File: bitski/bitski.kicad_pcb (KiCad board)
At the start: 2 copper layers, 90.8 x 42.4 mm, 6 parts, among them J1 USB_C_Receptacle, U1 ESP32-S3-MINI-1-N8, U2 BQ25185, U3 XC6206PxxxMR, U4 USBLC6-2SC6

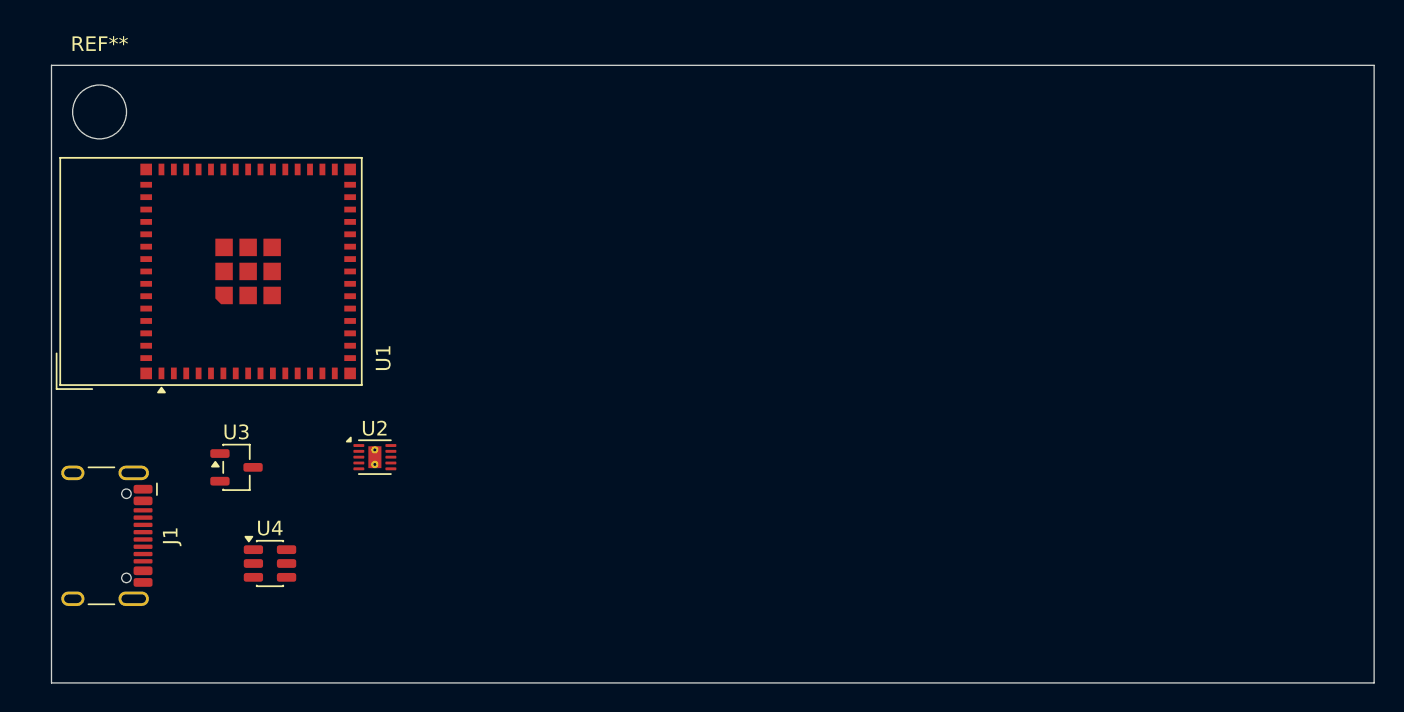
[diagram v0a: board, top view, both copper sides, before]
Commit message: made changes waow
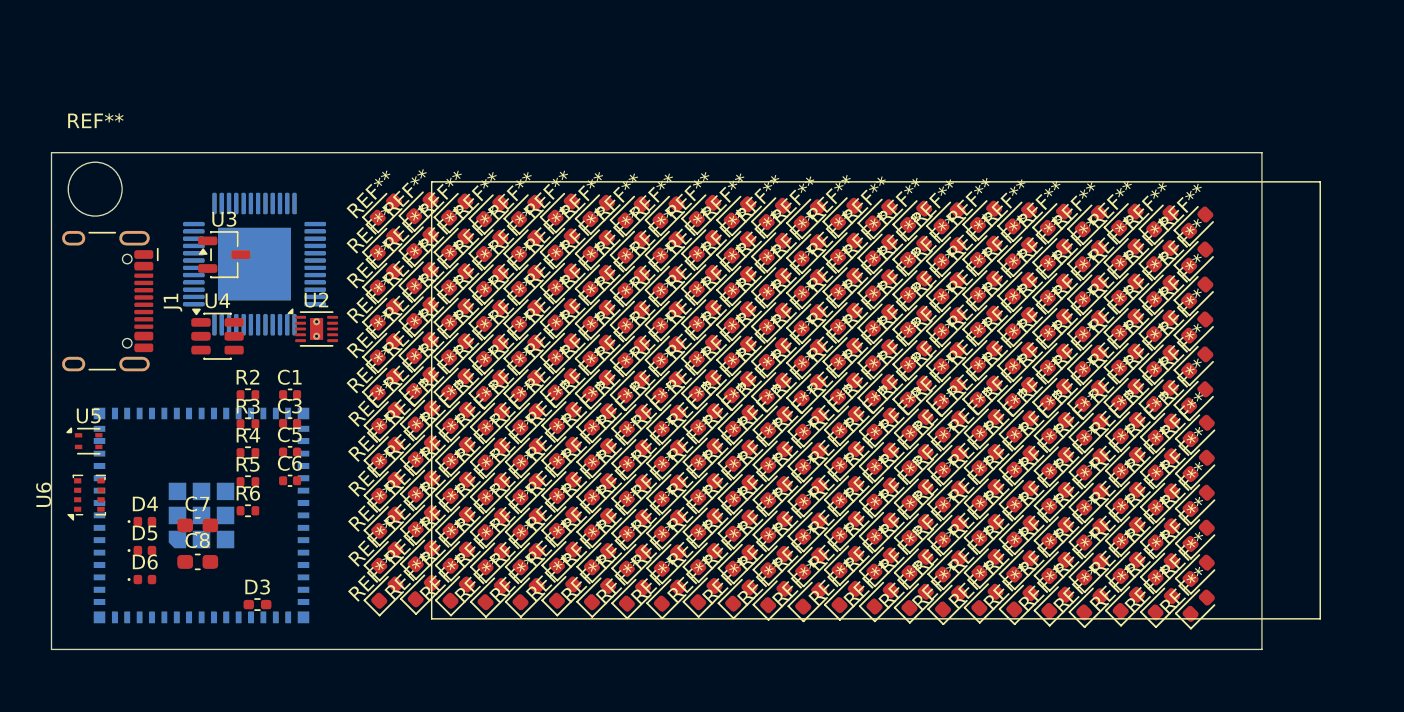
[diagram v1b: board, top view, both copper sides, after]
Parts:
- added C1: 10uF, Capacitor_SMD:C_0402_1005Metric, F.Cu at (114.0, 74.5)
- added C3: 1uF, Capacitor_SMD:C_0402_1005Metric, F.Cu at (114.0, 76.5)
- added C5: 1uF, Capacitor_SMD:C_0402_1005Metric, F.Cu at (114.0, 78.5)
- added C6: 1uF, Capacitor_SMD:C_0402_1005Metric, F.Cu at (114.0, 80.4)
- added C7: 0pF, Capacitor_SMD:C_0603_1608Metric_Pad1.08x0.95mm_HandSolder, F.Cu at (107.6, 83.5)
- added C8: 0pF, Capacitor_SMD:C_0603_1608Metric_Pad1.08x0.95mm_HandSolder, F.Cu at (107.6, 86.0)
- added D3: LED_45deg, Resistor_SMD:R_0402_1005Metric_Pad0.72x0.64mm_HandSolder, F.Cu at (111.7, 88.9)
- added D4: LED_45deg, LED_SMD:LED_0402_1005Metric, F.Cu at (104.0, 83.2)
- added D5: LED_45deg, LED_SMD:LED_0402_1005Metric, F.Cu at (104.0, 85.2)
- added D6: LED_45deg, LED_SMD:LED_0402_1005Metric, F.Cu at (104.0, 87.2)
- added R2: 5.1k, Resistor_SMD:R_0402_1005Metric, F.Cu at (111.1, 74.5)
- added R3: 5.1k, Resistor_SMD:R_0402_1005Metric, F.Cu at (111.1, 76.5)
- added R4: 10k, Resistor_SMD:R_0402_1005Metric, F.Cu at (111.1, 78.5)
- added R5: 33, Resistor_SMD:R_0402_1005Metric, F.Cu at (111.1, 80.5)
- added R6: 33, Resistor_SMD:R_0402_1005Metric, F.Cu at (111.1, 82.5)
- added REF**: LED_0603_1608Metric, LED_SMD:LED_0603_1608Metric, F.Cu at (157.0, 64.7)
- added REF**: LED_0603_1608Metric, LED_SMD:LED_0603_1608Metric, F.Cu at (154.7, 88.5)
- added REF**: LED_0603_1608Metric, LED_SMD:LED_0603_1608Metric, F.Cu at (132.8, 66.6)
- added REF**: LED_0603_1608Metric, LED_SMD:LED_0603_1608Metric, F.Cu at (169.0, 62.6)
- added REF**: LED_0603_1608Metric, LED_SMD:LED_0603_1608Metric, F.Cu at (135.3, 76.2)
- added REF**: LED_0603_1608Metric, LED_SMD:LED_0603_1608Metric, F.Cu at (147.3, 74.1)
- added REF**: LED_0603_1608Metric, LED_SMD:LED_0603_1608Metric, F.Cu at (144.9, 64.4)
- added REF**: LED_0603_1608Metric, LED_SMD:LED_0603_1608Metric, F.Cu at (120.7, 78.5)
- added REF**: LED_0603_1608Metric, LED_SMD:LED_0603_1608Metric, F.Cu at (123.2, 76.0)
- added REF**: LED_0603_1608Metric, LED_SMD:LED_0603_1608Metric, F.Cu at (152.2, 64.5)
- added REF**: LED_0603_1608Metric, LED_SMD:LED_0603_1608Metric, F.Cu at (176.3, 69.9)
- added REF**: LED_0603_1608Metric, LED_SMD:LED_0603_1608Metric, F.Cu at (152.3, 86.0)
- added REF**: LED_0603_1608Metric, LED_SMD:LED_0603_1608Metric, F.Cu at (127.9, 61.9)
- added REF**: LED_0603_1608Metric, LED_SMD:LED_0603_1608Metric, F.Cu at (176.4, 89.0)
- added REF**: LED_0603_1608Metric, LED_SMD:LED_0603_1608Metric, F.Cu at (152.2, 62.1)
- added REF**: LED_0603_1608Metric, LED_SMD:LED_0603_1608Metric, F.Cu at (169.0, 67.4)
- added REF**: LED_0603_1608Metric, LED_SMD:LED_0603_1608Metric, F.Cu at (123.2, 88.0)
- added REF**: LED_0603_1608Metric, LED_SMD:LED_0603_1608Metric, F.Cu at (169.1, 88.9)
- added REF**: LED_0603_1608Metric, LED_SMD:LED_0603_1608Metric, F.Cu at (142.5, 64.3)
- added REF**: LED_0603_1608Metric, LED_SMD:LED_0603_1608Metric, F.Cu at (154.6, 71.8)
- added REF**: LED_0603_1608Metric, LED_SMD:LED_0603_1608Metric, F.Cu at (140.1, 85.9)
- added REF**: LED_0603_1608Metric, LED_SMD:LED_0603_1608Metric, F.Cu at (142.5, 66.7)
- added REF**: LED_0603_1608Metric, LED_SMD:LED_0603_1608Metric, F.Cu at (174.0, 76.9)
- added REF**: LED_0603_1608Metric, LED_SMD:LED_0603_1608Metric, F.Cu at (137.7, 76.3)
- added REF**: LED_0603_1608Metric, LED_SMD:LED_0603_1608Metric, F.Cu at (149.7, 67.0)
- added REF**: LED_0603_1608Metric, LED_SMD:LED_0603_1608Metric, F.Cu at (142.6, 76.2)
- added REF**: LED_0603_1608Metric, LED_SMD:LED_0603_1608Metric, F.Cu at (161.8, 74.3)
- added REF**: LED_0603_1608Metric, LED_SMD:LED_0603_1608Metric, F.Cu at (125.5, 71.4)
- added REF**: LED_0603_1608Metric, LED_SMD:LED_0603_1608Metric, F.Cu at (120.6, 73.8)
- added REF**: LED_0603_1608Metric, LED_SMD:LED_0603_1608Metric, F.Cu at (164.3, 86.3)
- added REF**: LED_0603_1608Metric, LED_SMD:LED_0603_1608Metric, F.Cu at (125.6, 80.9)
- added REF**: LED_0603_1608Metric, LED_SMD:LED_0603_1608Metric, F.Cu at (145.0, 78.7)
- added REF**: LED_0603_1608Metric, LED_SMD:LED_0603_1608Metric, F.Cu at (161.8, 64.7)
- added REF**: LED_0603_1608Metric, LED_SMD:LED_0603_1608Metric, F.Cu at (159.4, 81.5)
- added REF**: LED_0603_1608Metric, LED_SMD:LED_0603_1608Metric, F.Cu at (135.2, 73.9)
- added REF**: LED_0603_1608Metric, LED_SMD:LED_0603_1608Metric, F.Cu at (166.7, 76.8)
- added REF**: LED_0603_1608Metric, LED_SMD:LED_0603_1608Metric, F.Cu at (161.8, 69.5)
- added REF**: LED_0603_1608Metric, LED_SMD:LED_0603_1608Metric, F.Cu at (171.5, 69.7)
- added REF**: LED_0603_1608Metric, LED_SMD:LED_0603_1608Metric, F.Cu at (176.3, 72.3)
- added REF**: LED_0603_1608Metric, LED_SMD:LED_0603_1608Metric, F.Cu at (123.2, 83.2)
- added REF**: LED_0603_1608Metric, LED_SMD:LED_0603_1608Metric, F.Cu at (154.7, 81.3)
- added REF**: LED_0603_1608Metric, LED_SMD:LED_0603_1608Metric, F.Cu at (161.8, 67.1)
- added REF**: LED_0603_1608Metric, LED_SMD:LED_0603_1608Metric, F.Cu at (149.7, 69.4)
- added REF**: LED_0603_1608Metric, LED_SMD:LED_0603_1608Metric, F.Cu at (142.6, 88.2)
- added REF**: LED_0603_1608Metric, LED_SMD:LED_0603_1608Metric, F.Cu at (176.3, 67.5)
- added REF**: LED_0603_1608Metric, LED_SMD:LED_0603_1608Metric, F.Cu at (157.1, 79.0)
- added REF**: LED_0603_1608Metric, LED_SMD:LED_0603_1608Metric, F.Cu at (125.6, 76.1)
- added REF**: LED_0603_1608Metric, LED_SMD:LED_0603_1608Metric, F.Cu at (176.4, 77.0)
- added REF**: LED_0603_1608Metric, LED_SMD:LED_0603_1608Metric, F.Cu at (159.4, 88.7)
- added REF**: LED_0603_1608Metric, LED_SMD:LED_0603_1608Metric, F.Cu at (137.7, 85.9)
- added REF**: LED_0603_1608Metric, LED_SMD:LED_0603_1608Metric, F.Cu at (161.8, 71.9)
- added REF**: LED_0603_1608Metric, LED_SMD:LED_0603_1608Metric, F.Cu at (144.9, 66.8)
- added REF**: LED_0603_1608Metric, LED_SMD:LED_0603_1608Metric, F.Cu at (130.3, 66.7)
- added REF**: LED_0603_1608Metric, LED_SMD:LED_0603_1608Metric, F.Cu at (144.9, 62.0)
- added REF**: LED_0603_1608Metric, LED_SMD:LED_0603_1608Metric, F.Cu at (164.2, 64.8)
- added REF**: LED_0603_1608Metric, LED_SMD:LED_0603_1608Metric, F.Cu at (140.1, 76.3)
- added REF**: LED_0603_1608Metric, LED_SMD:LED_0603_1608Metric, F.Cu at (157.1, 88.6)
- added REF**: LED_0603_1608Metric, LED_SMD:LED_0603_1608Metric, F.Cu at (123.1, 73.7)
- added REF**: LED_0603_1608Metric, LED_SMD:LED_0603_1608Metric, F.Cu at (135.3, 88.2)
- added REF**: LED_0603_1608Metric, LED_SMD:LED_0603_1608Metric, F.Cu at (135.2, 71.5)
- added REF**: LED_0603_1608Metric, LED_SMD:LED_0603_1608Metric, F.Cu at (132.9, 83.3)
- added REF**: LED_0603_1608Metric, LED_SMD:LED_0603_1608Metric, F.Cu at (171.6, 84.0)
- added REF**: LED_0603_1608Metric, LED_SMD:LED_0603_1608Metric, F.Cu at (149.8, 88.5)
- added REF**: LED_0603_1608Metric, LED_SMD:LED_0603_1608Metric, F.Cu at (174.0, 86.5)
- added REF**: LED_0603_1608Metric, LED_SMD:LED_0603_1608Metric, F.Cu at (176.3, 74.7)
- added REF**: LED_0603_1608Metric, LED_SMD:LED_0603_1608Metric, F.Cu at (132.8, 61.8)
- added REF**: LED_0603_1608Metric, LED_SMD:LED_0603_1608Metric, F.Cu at (173.9, 72.2)
- added REF**: LED_0603_1608Metric, LED_SMD:LED_0603_1608Metric, F.Cu at (145.0, 76.3)
- added REF**: LED_0603_1608Metric, LED_SMD:LED_0603_1608Metric, F.Cu at (171.6, 88.8)
- added REF**: LED_0603_1608Metric, LED_SMD:LED_0603_1608Metric, F.Cu at (169.1, 86.5)
- added REF**: LED_0603_1608Metric, LED_SMD:LED_0603_1608Metric, F.Cu at (130.4, 81.0)
- added REF**: LED_0603_1608Metric, LED_SMD:LED_0603_1608Metric, F.Cu at (164.2, 69.6)
- added REF**: LED_0603_1608Metric, LED_SMD:LED_0603_1608Metric, F.Cu at (154.7, 78.9)
- added REF**: LED_0603_1608Metric, LED_SMD:LED_0603_1608Metric, F.Cu at (137.6, 74.0)
- added REF**: LED_0603_1608Metric, LED_SMD:LED_0603_1608Metric, F.Cu at (176.3, 65.1)
- added REF**: LED_0603_1608Metric, LED_SMD:LED_0603_1608Metric, F.Cu at (147.4, 78.8)
- added REF**: LED_0603_1608Metric, LED_SMD:LED_0603_1608Metric, F.Cu at (176.4, 81.8)
- added REF**: LED_0603_1608Metric, LED_SMD:LED_0603_1608Metric, F.Cu at (173.9, 62.6)
- added REF**: LED_0603_1608Metric, LED_SMD:LED_0603_1608Metric, F.Cu at (164.3, 81.5)
- added REF**: LED_0603_1608Metric, LED_SMD:LED_0603_1608Metric, F.Cu at (137.7, 88.3)
- added REF**: LED_0603_1608Metric, LED_SMD:LED_0603_1608Metric, F.Cu at (159.3, 69.6)
- added REF**: LED_0603_1608Metric, LED_SMD:LED_0603_1608Metric, F.Cu at (135.3, 83.4)
- added REF**: LED_0603_1608Metric, LED_SMD:LED_0603_1608Metric, F.Cu at (132.9, 85.7)
- added REF**: LED_0603_1608Metric, LED_SMD:LED_0603_1608Metric, F.Cu at (135.2, 66.7)
- added REF**: LED_0603_1608Metric, LED_SMD:LED_0603_1608Metric, F.Cu at (157.1, 83.8)
- added REF**: LED_0603_1608Metric, LED_SMD:LED_0603_1608Metric, F.Cu at (157.0, 62.3)
- added REF**: LED_0603_1608Metric, LED_SMD:LED_0603_1608Metric, F.Cu at (135.2, 61.9)
- added REF**: LED_0603_1608Metric, LED_SMD:LED_0603_1608Metric, F.Cu at (166.6, 72.1)
- added REF**: LED_0603_1608Metric, LED_SMD:LED_0603_1608Metric, F.Cu at (169.0, 69.8)
- added REF**: LED_0603_1608Metric, LED_SMD:LED_0603_1608Metric, F.Cu at (173.9, 67.4)
- added REF**: LED_0603_1608Metric, LED_SMD:LED_0603_1608Metric, F.Cu at (140.0, 69.2)
- added REF**: LED_0603_1608Metric, LED_SMD:LED_0603_1608Metric, F.Cu at (120.6, 69.0)
- added REF**: LED_0603_1608Metric, LED_SMD:LED_0603_1608Metric, F.Cu at (140.0, 62.0)
- added REF**: LED_0603_1608Metric, LED_SMD:LED_0603_1608Metric, F.Cu at (142.6, 83.4)
- added REF**: LED_0603_1608Metric, LED_SMD:LED_0603_1608Metric, F.Cu at (166.6, 62.5)
- added REF**: LED_0603_1608Metric, LED_SMD:LED_0603_1608Metric, F.Cu at (164.2, 62.4)
- added REF**: LED_0603_1608Metric, LED_SMD:LED_0603_1608Metric, F.Cu at (171.6, 76.8)
- added REF**: LED_0603_1608Metric, LED_SMD:LED_0603_1608Metric, F.Cu at (142.6, 81.0)
- added REF**: LED_0603_1608Metric, LED_SMD:LED_0603_1608Metric, F.Cu at (147.4, 88.4)
- added REF**: LED_0603_1608Metric, LED_SMD:LED_0603_1608Metric, F.Cu at (128.0, 78.6)
- added REF**: LED_0603_1608Metric, LED_SMD:LED_0603_1608Metric, F.Cu at (130.4, 83.4)
- added REF**: LED_0603_1608Metric, LED_SMD:LED_0603_1608Metric, F.Cu at (120.7, 76.1)
- added REF**: LED_0603_1608Metric, LED_SMD:LED_0603_1608Metric, F.Cu at (171.5, 72.1)
- added REF**: LED_0603_1608Metric, LED_SMD:LED_0603_1608Metric, F.Cu at (159.4, 76.7)
- added REF**: LED_0603_1608Metric, LED_SMD:LED_0603_1608Metric, F.Cu at (161.9, 88.6)
- added REF**: LED_0603_1608Metric, LED_SMD:LED_0603_1608Metric, F.Cu at (171.5, 67.3)
- added REF**: LED_0603_1608Metric, LED_SMD:LED_0603_1608Metric, F.Cu at (140.0, 71.6)
- added REF**: LED_0603_1608Metric, LED_SMD:LED_0603_1608Metric, F.Cu at (125.5, 61.8)
- added REF**: LED_0603_1608Metric, LED_SMD:LED_0603_1608Metric, F.Cu at (159.4, 79.1)
- added REF**: LED_0603_1608Metric, LED_SMD:LED_0603_1608Metric, F.Cu at (174.0, 81.7)
- added REF**: LED_0603_1608Metric, LED_SMD:LED_0603_1608Metric, F.Cu at (176.4, 79.4)
- added REF**: LED_0603_1608Metric, LED_SMD:LED_0603_1608Metric, F.Cu at (130.3, 64.3)
- added REF**: LED_0603_1608Metric, LED_SMD:LED_0603_1608Metric, F.Cu at (169.1, 81.7)
- added REF**: LED_0603_1608Metric, LED_SMD:LED_0603_1608Metric, F.Cu at (130.3, 71.5)
- added REF**: LED_0603_1608Metric, LED_SMD:LED_0603_1608Metric, F.Cu at (149.8, 78.9)
- added REF**: LED_0603_1608Metric, LED_SMD:LED_0603_1608Metric, F.Cu at (127.9, 71.5)
- added REF**: LED_0603_1608Metric, LED_SMD:LED_0603_1608Metric, F.Cu at (145.0, 81.1)
- added REF**: LED_0603_1608Metric, LED_SMD:LED_0603_1608Metric, F.Cu at (166.7, 84.0)
- added REF**: LED_0603_1608Metric, LED_SMD:LED_0603_1608Metric, F.Cu at (174.0, 84.1)
- added REF**: LED_0603_1608Metric, LED_SMD:LED_0603_1608Metric, F.Cu at (135.2, 69.1)
- added REF**: LED_0603_1608Metric, LED_SMD:LED_0603_1608Metric, F.Cu at (154.6, 67.0)
- added REF**: LED_0603_1608Metric, LED_SMD:LED_0603_1608Metric, F.Cu at (154.6, 62.2)
- added REF**: LED_0603_1608Metric, LED_SMD:LED_0603_1608Metric, F.Cu at (149.7, 62.2)
- added REF**: LED_0603_1608Metric, LED_SMD:LED_0603_1608Metric, F.Cu at (132.8, 71.4)
- added REF**: LED_0603_1608Metric, LED_SMD:LED_0603_1608Metric, F.Cu at (137.7, 81.1)
- added REF**: LED_0603_1608Metric, LED_SMD:LED_0603_1608Metric, F.Cu at (157.0, 69.5)
- added REF**: LED_0603_1608Metric, LED_SMD:LED_0603_1608Metric, F.Cu at (159.3, 67.2)
- added REF**: LED_0603_1608Metric, LED_SMD:LED_0603_1608Metric, F.Cu at (130.3, 61.9)
- added REF**: LED_0603_1608Metric, LED_SMD:LED_0603_1608Metric, F.Cu at (147.4, 86.0)
- added REF**: LED_0603_1608Metric, LED_SMD:LED_0603_1608Metric, F.Cu at (125.6, 88.1)
- added REF**: LED_0603_1608Metric, LED_SMD:LED_0603_1608Metric, F.Cu at (176.3, 62.7)
- added REF**: LED_0603_1608Metric, LED_SMD:LED_0603_1608Metric, F.Cu at (164.2, 74.4)
- added REF**: LED_0603_1608Metric, LED_SMD:LED_0603_1608Metric, F.Cu at (123.1, 68.9)
- added REF**: LED_0603_1608Metric, LED_SMD:LED_0603_1608Metric, F.Cu at (171.5, 62.5)
- added REF**: LED_0603_1608Metric, LED_SMD:LED_0603_1608Metric, F.Cu at (140.0, 74.0)
- added REF**: LED_0603_1608Metric, LED_SMD:LED_0603_1608Metric, F.Cu at (169.0, 74.6)
- added REF**: LED_0603_1608Metric, LED_SMD:LED_0603_1608Metric, F.Cu at (173.9, 69.8)
- added REF**: LED_0603_1608Metric, LED_SMD:LED_0603_1608Metric, F.Cu at (169.0, 65.0)
- added REF**: LED_0603_1608Metric, LED_SMD:LED_0603_1608Metric, F.Cu at (142.5, 73.9)
- added REF**: LED_0603_1608Metric, LED_SMD:LED_0603_1608Metric, F.Cu at (125.6, 78.5)
- added REF**: LED_0603_1608Metric, LED_SMD:LED_0603_1608Metric, F.Cu at (166.6, 74.5)
- added REF**: LED_0603_1608Metric, LED_SMD:LED_0603_1608Metric, F.Cu at (169.0, 72.2)
- added REF**: LED_0603_1608Metric, LED_SMD:LED_0603_1608Metric, F.Cu at (132.8, 64.2)
- added REF**: LED_0603_1608Metric, LED_SMD:LED_0603_1608Metric, F.Cu at (174.0, 79.3)
- added REF**: LED_0603_1608Metric, LED_SMD:LED_0603_1608Metric, F.Cu at (147.4, 76.4)
- added REF**: LED_0603_1608Metric, LED_SMD:LED_0603_1608Metric, F.Cu at (147.3, 64.5)
- added REF**: LED_0603_1608Metric, LED_SMD:LED_0603_1608Metric, F.Cu at (127.9, 66.7)
- added REF**: LED_0603_1608Metric, LED_SMD:LED_0603_1608Metric, F.Cu at (120.6, 61.8)
- added REF**: LED_0603_1608Metric, LED_SMD:LED_0603_1608Metric, F.Cu at (142.5, 69.1)
- added REF**: LED_0603_1608Metric, LED_SMD:LED_0603_1608Metric, F.Cu at (169.1, 79.3)
- added REF**: LED_0603_1608Metric, LED_SMD:LED_0603_1608Metric, F.Cu at (171.5, 64.9)
- added REF**: LED_0603_1608Metric, LED_SMD:LED_0603_1608Metric, F.Cu at (130.4, 88.2)
- added REF**: LED_0603_1608Metric, LED_SMD:LED_0603_1608Metric, F.Cu at (123.2, 85.6)
- added REF**: LED_0603_1608Metric, LED_SMD:LED_0603_1608Metric, F.Cu at (149.8, 81.3)
- added REF**: LED_0603_1608Metric, LED_SMD:LED_0603_1608Metric, F.Cu at (174.0, 88.9)
- added REF**: LED_0603_1608Metric, LED_SMD:LED_0603_1608Metric, F.Cu at (154.7, 76.5)
- added REF**: LED_0603_1608Metric, LED_SMD:LED_0603_1608Metric, F.Cu at (135.3, 78.6)
- added REF**: LED_0603_1608Metric, LED_SMD:LED_0603_1608Metric, F.Cu at (157.1, 76.6)
- added REF**: LED_0603_1608Metric, LED_SMD:LED_0603_1608Metric, F.Cu at (161.9, 76.6)
- added REF**: LED_0603_1608Metric, LED_SMD:LED_0603_1608Metric, F.Cu at (137.6, 66.8)
- added REF**: LED_0603_1608Metric, LED_SMD:LED_0603_1608Metric, F.Cu at (149.7, 64.6)
- added REF**: LED_0603_1608Metric, LED_SMD:LED_0603_1608Metric, F.Cu at (147.4, 83.6)
- added REF**: LED_0603_1608Metric, LED_SMD:LED_0603_1608Metric, F.Cu at (132.9, 88.1)
- added REF**: LED_0603_1608Metric, LED_SMD:LED_0603_1608Metric, F.Cu at (142.6, 78.6)
- added REF**: LED_0603_1608Metric, LED_SMD:LED_0603_1608Metric, F.Cu at (149.8, 86.1)
- added REF**: LED_0603_1608Metric, LED_SMD:LED_0603_1608Metric, F.Cu at (142.6, 85.8)
- added REF**: LED_0603_1608Metric, LED_SMD:LED_0603_1608Metric, F.Cu at (171.5, 74.5)
- added REF**: LED_0603_1608Metric, LED_SMD:LED_0603_1608Metric, F.Cu at (123.1, 61.7)
- added REF**: LED_0603_1608Metric, LED_SMD:LED_0603_1608Metric, F.Cu at (164.3, 76.7)
- added REF**: LED_0603_1608Metric, LED_SMD:LED_0603_1608Metric, F.Cu at (159.3, 72.0)
- added REF**: LED_0603_1608Metric, LED_SMD:LED_0603_1608Metric, F.Cu at (135.2, 64.3)
- added REF**: LED_0603_1608Metric, LED_SMD:LED_0603_1608Metric, F.Cu at (128.0, 83.4)
- added REF**: LED_0603_1608Metric, LED_SMD:LED_0603_1608Metric, F.Cu at (157.0, 74.3)
- added REF**: LED_0603_1608Metric, LED_SMD:LED_0603_1608Metric, F.Cu at (159.3, 62.4)
- added REF**: LED_0603_1608Metric, LED_SMD:LED_0603_1608Metric, F.Cu at (135.3, 81.0)
- added REF**: LED_0603_1608Metric, LED_SMD:LED_0603_1608Metric, F.Cu at (125.5, 64.2)
- added REF**: LED_0603_1608Metric, LED_SMD:LED_0603_1608Metric, F.Cu at (157.1, 86.2)
- added REF**: LED_0603_1608Metric, LED_SMD:LED_0603_1608Metric, F.Cu at (140.0, 64.4)
- added REF**: LED_0603_1608Metric, LED_SMD:LED_0603_1608Metric, F.Cu at (137.7, 83.5)
- added REF**: LED_0603_1608Metric, LED_SMD:LED_0603_1608Metric, F.Cu at (140.1, 81.1)
- added REF**: LED_0603_1608Metric, LED_SMD:LED_0603_1608Metric, F.Cu at (132.8, 69.0)
- added REF**: LED_0603_1608Metric, LED_SMD:LED_0603_1608Metric, F.Cu at (149.8, 83.7)
- added REF**: LED_0603_1608Metric, LED_SMD:LED_0603_1608Metric, F.Cu at (142.5, 71.5)
- added REF**: LED_0603_1608Metric, LED_SMD:LED_0603_1608Metric, F.Cu at (152.2, 71.7)
- added REF**: LED_0603_1608Metric, LED_SMD:LED_0603_1608Metric, F.Cu at (147.3, 71.7)
- added REF**: LED_0603_1608Metric, LED_SMD:LED_0603_1608Metric, F.Cu at (152.3, 76.4)
- added REF**: LED_0603_1608Metric, LED_SMD:LED_0603_1608Metric, F.Cu at (161.9, 81.4)
- added REF**: LED_0603_1608Metric, LED_SMD:LED_0603_1608Metric, F.Cu at (166.7, 88.8)
- added REF**: LED_0603_1608Metric, LED_SMD:LED_0603_1608Metric, F.Cu at (152.3, 83.6)
- added REF**: LED_0603_1608Metric, LED_SMD:LED_0603_1608Metric, F.Cu at (154.6, 69.4)
- added REF**: LED_0603_1608Metric, LED_SMD:LED_0603_1608Metric, F.Cu at (137.6, 69.2)
- added REF**: LED_0603_1608Metric, LED_SMD:LED_0603_1608Metric, F.Cu at (149.7, 74.2)
- added REF**: LED_0603_1608Metric, LED_SMD:LED_0603_1608Metric, F.Cu at (173.9, 65.0)
- added REF**: LED_0603_1608Metric, LED_SMD:LED_0603_1608Metric, F.Cu at (157.0, 71.9)
- added REF**: LED_0603_1608Metric, LED_SMD:LED_0603_1608Metric, F.Cu at (176.4, 84.2)
- added REF**: LED_0603_1608Metric, LED_SMD:LED_0603_1608Metric, F.Cu at (120.6, 64.2)
- added REF**: LED_0603_1608Metric, LED_SMD:LED_0603_1608Metric, F.Cu at (166.6, 67.3)
- added REF**: LED_0603_1608Metric, LED_SMD:LED_0603_1608Metric, F.Cu at (152.3, 78.8)
- added REF**: LED_0603_1608Metric, LED_SMD:LED_0603_1608Metric, F.Cu at (128.0, 81.0)
- added REF**: LED_0603_1608Metric, LED_SMD:LED_0603_1608Metric, F.Cu at (144.9, 71.6)
- added REF**: LED_0603_1608Metric, LED_SMD:LED_0603_1608Metric, F.Cu at (152.3, 88.4)
- added REF**: LED_0603_1608Metric, LED_SMD:LED_0603_1608Metric, F.Cu at (159.3, 74.4)
- added REF**: LED_0603_1608Metric, LED_SMD:LED_0603_1608Metric, F.Cu at (130.4, 78.6)
- added REF**: LED_0603_1608Metric, LED_SMD:LED_0603_1608Metric, F.Cu at (145.0, 83.5)
- added REF**: LED_0603_1608Metric, LED_SMD:LED_0603_1608Metric, F.Cu at (125.5, 66.6)
- added REF**: LED_0603_1608Metric, LED_SMD:LED_0603_1608Metric, F.Cu at (120.7, 88.1)
- added REF**: LED_0603_1608Metric, LED_SMD:LED_0603_1608Metric, F.Cu at (132.9, 80.9)
- added REF**: LED_0603_1608Metric, LED_SMD:LED_0603_1608Metric, F.Cu at (149.8, 76.5)
- added REF**: LED_0603_1608Metric, LED_SMD:LED_0603_1608Metric, F.Cu at (132.8, 73.8)
- added REF**: LED_0603_1608Metric, LED_SMD:LED_0603_1608Metric, F.Cu at (137.6, 71.6)
- added REF**: LED_0603_1608Metric, LED_SMD:LED_0603_1608Metric, F.Cu at (145.0, 85.9)
- added REF**: LED_0603_1608Metric, LED_SMD:LED_0603_1608Metric, F.Cu at (152.2, 69.3)
- added REF**: LED_0603_1608Metric, LED_SMD:LED_0603_1608Metric, F.Cu at (161.9, 79.0)
- added REF**: LED_0603_1608Metric, LED_SMD:LED_0603_1608Metric, F.Cu at (140.1, 83.5)
- added REF**: LED_0603_1608Metric, LED_SMD:LED_0603_1608Metric, F.Cu at (169.1, 84.1)
- added REF**: LED_0603_1608Metric, LED_SMD:LED_0603_1608Metric, F.Cu at (166.7, 86.4)
- added REF**: LED_0603_1608Metric, LED_SMD:LED_0603_1608Metric, F.Cu at (171.6, 79.2)
- added REF**: LED_0603_1608Metric, LED_SMD:LED_0603_1608Metric, F.Cu at (152.3, 81.2)
- added REF**: LED_0603_1608Metric, LED_SMD:LED_0603_1608Metric, F.Cu at (154.7, 83.7)
- added REF**: LED_0603_1608Metric, LED_SMD:LED_0603_1608Metric, F.Cu at (135.3, 85.8)
- added REF**: LED_0603_1608Metric, LED_SMD:LED_0603_1608Metric, F.Cu at (157.0, 67.1)
- added REF**: LED_0603_1608Metric, LED_SMD:LED_0603_1608Metric, F.Cu at (147.4, 81.2)
- added REF**: LED_0603_1608Metric, LED_SMD:LED_0603_1608Metric, F.Cu at (144.9, 69.2)
- added REF**: LED_0603_1608Metric, LED_SMD:LED_0603_1608Metric, F.Cu at (164.3, 83.9)
- added REF**: LED_0603_1608Metric, LED_SMD:LED_0603_1608Metric, F.Cu at (125.6, 83.3)
- added REF**: LED_0603_1608Metric, LED_SMD:LED_0603_1608Metric, F.Cu at (152.2, 66.9)
- added REF**: LED_0603_1608Metric, LED_SMD:LED_0603_1608Metric, F.Cu at (123.1, 66.5)
- added REF**: LED_0603_1608Metric, LED_SMD:LED_0603_1608Metric, F.Cu at (166.7, 81.6)
- added REF**: LED_0603_1608Metric, LED_SMD:LED_0603_1608Metric, F.Cu at (159.4, 83.9)
- added REF**: LED_0603_1608Metric, LED_SMD:LED_0603_1608Metric, F.Cu at (147.3, 66.9)
- added REF**: LED_0603_1608Metric, LED_SMD:LED_0603_1608Metric, F.Cu at (127.9, 69.1)
- added REF**: LED_0603_1608Metric, LED_SMD:LED_0603_1608Metric, F.Cu at (130.4, 76.2)
- added REF**: LED_0603_1608Metric, LED_SMD:LED_0603_1608Metric, F.Cu at (154.6, 74.2)
- added REF**: LED_0603_1608Metric, LED_SMD:LED_0603_1608Metric, F.Cu at (145.0, 88.3)
- added REF**: LED_0603_1608Metric, LED_SMD:LED_0603_1608Metric, F.Cu at (171.6, 86.4)
- added REF**: LED_0603_1608Metric, LED_SMD:LED_0603_1608Metric, F.Cu at (173.9, 74.6)
- added REF**: LED_0603_1608Metric, LED_SMD:LED_0603_1608Metric, F.Cu at (120.7, 80.9)
- added REF**: LED_0603_1608Metric, LED_SMD:LED_0603_1608Metric, F.Cu at (127.9, 73.9)
- added REF**: LED_0603_1608Metric, LED_SMD:LED_0603_1608Metric, F.Cu at (157.1, 81.4)
- added REF**: LED_0603_1608Metric, LED_SMD:LED_0603_1608Metric, F.Cu at (147.3, 69.3)
- added REF**: LED_0603_1608Metric, LED_SMD:LED_0603_1608Metric, F.Cu at (128.0, 76.2)
- added REF**: LED_0603_1608Metric, LED_SMD:LED_0603_1608Metric, F.Cu at (140.0, 66.8)
- added REF**: LED_0603_1608Metric, LED_SMD:LED_0603_1608Metric, F.Cu at (123.2, 80.8)
- added REF**: LED_0603_1608Metric, LED_SMD:LED_0603_1608Metric, F.Cu at (130.3, 73.9)
- added REF**: LED_0603_1608Metric, LED_SMD:LED_0603_1608Metric, F.Cu at (120.7, 85.7)
- added REF**: LED_0603_1608Metric, LED_SMD:LED_0603_1608Metric, F.Cu at (140.1, 88.3)
- added REF**: LED_0603_1608Metric, LED_SMD:LED_0603_1608Metric, F.Cu at (159.3, 64.8)
- added REF**: LED_0603_1608Metric, LED_SMD:LED_0603_1608Metric, F.Cu at (127.9, 64.3)
- added REF**: LED_0603_1608Metric, LED_SMD:LED_0603_1608Metric, F.Cu at (164.3, 88.7)
- added REF**: LED_0603_1608Metric, LED_SMD:LED_0603_1608Metric, F.Cu at (132.9, 76.1)
- added REF**: LED_0603_1608Metric, LED_SMD:LED_0603_1608Metric, F.Cu at (140.1, 78.7)
- added REF**: LED_0603_1608Metric, LED_SMD:LED_0603_1608Metric, F.Cu at (137.6, 62.0)
- added REF**: LED_0603_1608Metric, LED_SMD:LED_0603_1608Metric, F.Cu at (149.7, 71.8)
- added REF**: LED_0603_1608Metric, LED_SMD:LED_0603_1608Metric, F.Cu at (166.6, 69.7)
- added REF**: LED_0603_1608Metric, LED_SMD:LED_0603_1608Metric, F.Cu at (164.3, 79.1)
- added REF**: LED_0603_1608Metric, LED_SMD:LED_0603_1608Metric, F.Cu at (154.6, 64.6)
- added REF**: LED_0603_1608Metric, LED_SMD:LED_0603_1608Metric, F.Cu at (120.6, 66.6)
- added REF**: LED_0603_1608Metric, LED_SMD:LED_0603_1608Metric, F.Cu at (125.6, 85.7)
- added REF**: LED_0603_1608Metric, LED_SMD:LED_0603_1608Metric, F.Cu at (130.4, 85.8)
- added REF**: LED_0603_1608Metric, LED_SMD:LED_0603_1608Metric, F.Cu at (128.0, 88.2)
- added REF**: LED_0603_1608Metric, LED_SMD:LED_0603_1608Metric, F.Cu at (152.2, 74.1)
- added REF**: LED_0603_1608Metric, LED_SMD:LED_0603_1608Metric, F.Cu at (120.7, 83.3)
- added REF**: LED_0603_1608Metric, LED_SMD:LED_0603_1608Metric, F.Cu at (164.2, 67.2)
- added REF**: LED_0603_1608Metric, LED_SMD:LED_0603_1608Metric, F.Cu at (161.9, 86.2)
- added REF**: LED_0603_1608Metric, LED_SMD:LED_0603_1608Metric, F.Cu at (147.3, 62.1)
- added REF**: LED_0603_1608Metric, LED_SMD:LED_0603_1608Metric, F.Cu at (125.5, 69.0)
- added REF**: LED_0603_1608Metric, LED_SMD:LED_0603_1608Metric, F.Cu at (123.1, 71.3)
- added REF**: LED_0603_1608Metric, LED_SMD:LED_0603_1608Metric, F.Cu at (176.4, 86.6)
- added REF**: LED_0603_1608Metric, LED_SMD:LED_0603_1608Metric, F.Cu at (130.3, 69.1)
- added REF**: LED_0603_1608Metric, LED_SMD:LED_0603_1608Metric, F.Cu at (154.7, 86.1)
- added REF**: LED_0603_1608Metric, LED_SMD:LED_0603_1608Metric, F.Cu at (137.6, 64.4)
- added REF**: LED_0603_1608Metric, LED_SMD:LED_0603_1608Metric, F.Cu at (128.0, 85.8)
- added REF**: LED_0603_1608Metric, LED_SMD:LED_0603_1608Metric, F.Cu at (123.2, 78.4)
- added REF**: LED_0603_1608Metric, LED_SMD:LED_0603_1608Metric, F.Cu at (161.8, 62.3)
- added REF**: LED_0603_1608Metric, LED_SMD:LED_0603_1608Metric, F.Cu at (144.9, 74.0)
- added REF**: LED_0603_1608Metric, LED_SMD:LED_0603_1608Metric, F.Cu at (159.4, 86.3)
- added REF**: LED_0603_1608Metric, LED_SMD:LED_0603_1608Metric, F.Cu at (125.5, 73.8)
- added REF**: LED_0603_1608Metric, LED_SMD:LED_0603_1608Metric, F.Cu at (137.7, 78.7)
- added REF**: LED_0603_1608Metric, LED_SMD:LED_0603_1608Metric, F.Cu at (166.6, 64.9)
- added REF**: LED_0603_1608Metric, LED_SMD:LED_0603_1608Metric, F.Cu at (132.9, 78.5)
- added REF**: LED_0603_1608Metric, LED_SMD:LED_0603_1608Metric, F.Cu at (120.6, 71.4)
- added REF**: LED_0603_1608Metric, LED_SMD:LED_0603_1608Metric, F.Cu at (171.6, 81.6)
- added REF**: LED_0603_1608Metric, LED_SMD:LED_0603_1608Metric, F.Cu at (123.1, 64.1)
- added REF**: LED_0603_1608Metric, LED_SMD:LED_0603_1608Metric, F.Cu at (166.7, 79.2)
- added REF**: LED_0603_1608Metric, LED_SMD:LED_0603_1608Metric, F.Cu at (161.9, 83.8)
- added REF**: LED_0603_1608Metric, LED_SMD:LED_0603_1608Metric, F.Cu at (142.5, 61.9)
- added REF**: LED_0603_1608Metric, LED_SMD:LED_0603_1608Metric, F.Cu at (164.2, 72.0)
- added REF**: LED_0603_1608Metric, LED_SMD:LED_0603_1608Metric, F.Cu at (169.1, 76.9)
- added U5: GXHT40AD, Sensor_Humidity:Sensirion_DFN-4_1.5x1.5mm_P0.8mm_SHT4x_NoCentralPad, F.Cu at (100.2, 77.7)
- added U6: BMP280, Package_LGA:Bosch_LGA-8_2x2.5mm_P0.65mm_ClockwisePinNumbering, F.Cu at (100.2, 81.4)
- added U7: IS31FL3733-TQ, Package_QFP:TQFP-48-1EP_7x7mm_P0.5mm_EP5x5mm, B.Cu at (111.5, 65.5)
- U1: moved to B.Cu
- moved U1 19.3 mm to (107.9, 85.3), turned to 0 degrees
- moved J1 16.1 mm to (100.2, 68.1)
- moved U4 16.0 mm to (109.0, 70.5)
- moved U3 14.6 mm to (109.5, 64.9)
- moved U2 9.67 mm to (115.8, 70.0)
- moved REF** 5.31 mm to (100.6, 60.4)
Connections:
- U3 pad 2: +3V3 -> Net-(SW6-B)
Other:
- board size 90.8 x 42.4 mm -> 83.1 x 34.1 mm
